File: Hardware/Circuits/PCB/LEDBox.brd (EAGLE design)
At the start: 28 x 28 mm, 19 parts

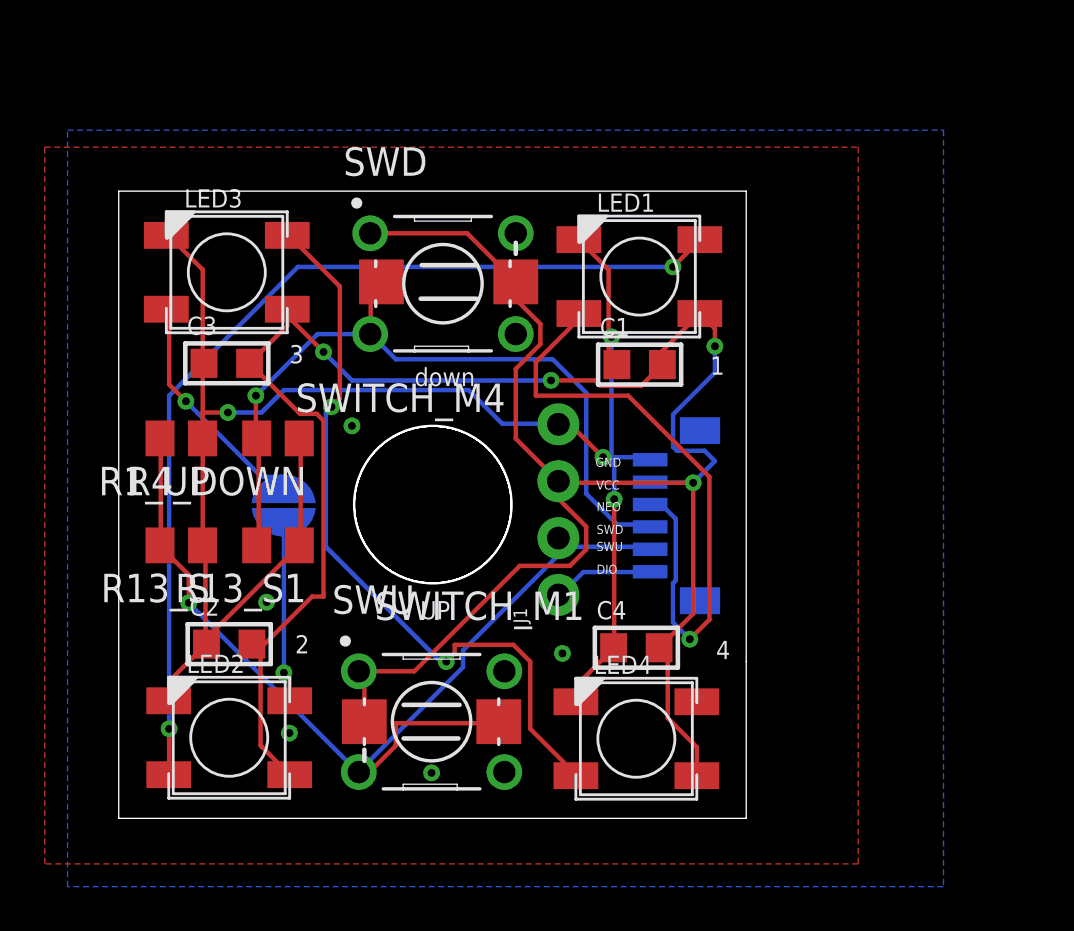
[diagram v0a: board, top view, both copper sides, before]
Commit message: update circuits
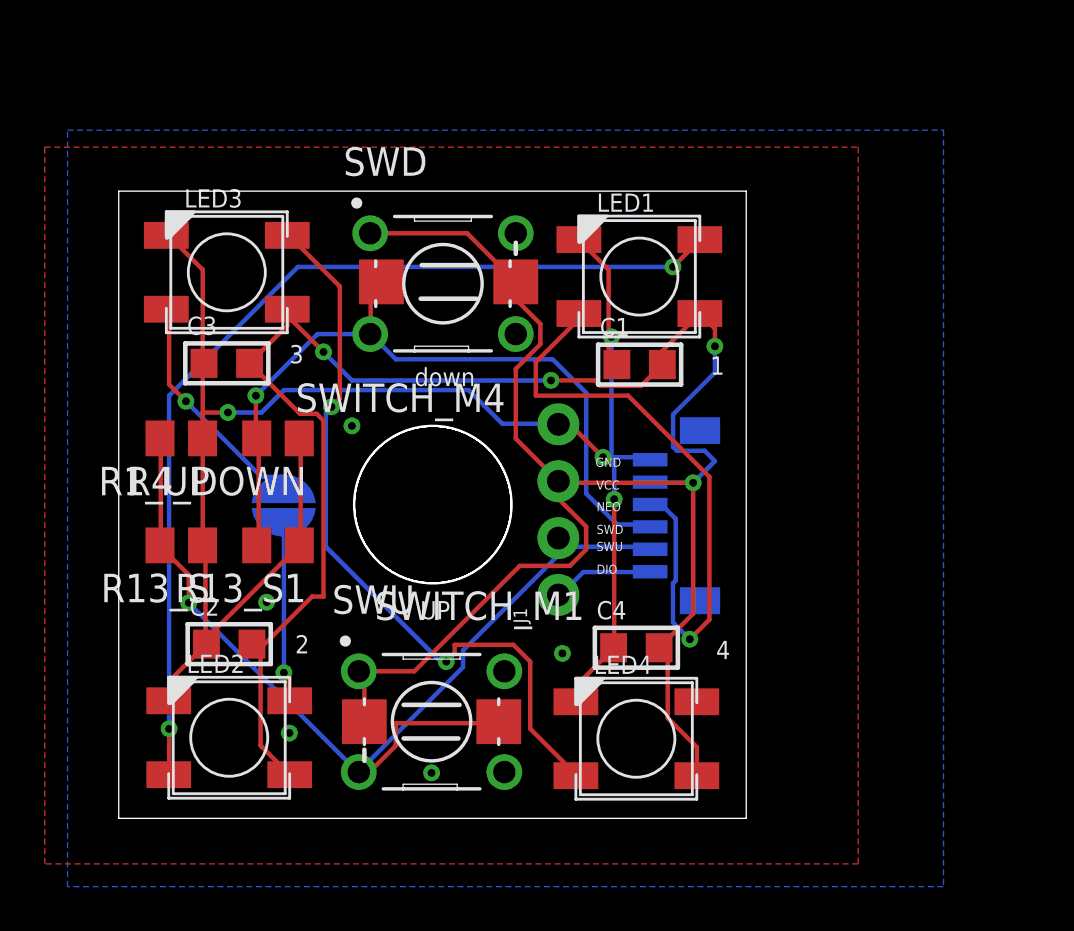
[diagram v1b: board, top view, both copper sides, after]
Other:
- outline, holes or cut-outs redrawn
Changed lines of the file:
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@@
 <drawing>
 <settings>
-<setting alwaysvectorfont="yes"/>
+<setting alwaysvectorfont="no"/>
 <setting verticaltext="up"/>
 </settings>
 <grid distance="10" unitdist="mil" unit="mm" style="lines" multiple="1" display="no" altdistance="1" altunitdist="mil" altunit="mm"/>
 <layers>
-<layer number="1" name="Top" color="4" fill="1" visible="yes" active="yes"/>
+<layer number="1" name="Top" color="4" fill="1" visible="no" active="yes"/>
 <layer number="2" name="Route2" color="16" fill="1" visible="no" active="no"/>
 <layer number="3" name="Route3" color="17" fill="1" visible="no" active="no"/>
@@
 <layer number="14" name="Route14" color="22" fill="1" visible="no" active="no"/>
 <layer number="15" name="Route15" color="23" fill="1" visible="no" active="no"/>
-<layer number="16" name="Bottom" color="1" fill="1" visible="yes" active="yes"/>
+<layer number="16" name="Bottom" color="1" fill="1" visible="no" active="yes"/>
 <layer number="17" name="Pads" color="2" fill="1" visible="yes" active="yes"/>
-<layer number="18" name="Vias" color="2" fill="1" visible="yes" active="yes"/>
-<layer number="19" name="Unrouted" color="6" fill="1" visible="yes" active="yes"/>
+<layer number="18" name="Vias" color="2" fill="1" visible="no" active="yes"/>
+<layer number="19" name="Unrouted" color="6" fill="1" visible="no" active="yes"/>
 <layer number="20" name="Dimension" color="24" fill="1" visible="yes" active="yes"/>
-<layer number="21" name="tPlace" color="7" fill="1" visible="yes" active="yes"/>
+<layer number="21" name="tPlace" color="7" fill="1" visible="no" active="yes"/>
 <layer number="22" name="bPlace" color="7" fill="1" visible="yes" active="yes"/>
-<layer number="23" name="tOrigins" color="15" fill="1" visible="yes" active="yes"/>
-<layer number="24" name="bOrigins" color="15" fill="1" visible="yes" active="yes"/>
-<layer number="25" name="tNames" color="7" fill="1" visible="yes" active="yes"/>
-<layer number="26" name="bNames" color="7" fill="1" visible="yes" active="yes"/>
+<layer number="23" name="tOrigins" color="15" fill="1" visible="no" active="yes"/>
+<layer number="24" name="bOrigins" color="15" fill="1" visible="no" active="yes"/>
+<layer number="25" name="tNames" color="7" fill="1" visible="no" active="yes"/>
+<layer number="26" name="bNames" color="7" fill="1" visible="no" active="yes"/>
 <layer number="27" name="tValues" color="7" fill="1" visible="no" active="yes"/>
 <layer number="28" name="bValues" color="7" fill="1" visible="no" active="yes"/>
@@
 <layer number="43" name="vRestrict" color="2" fill="10" visible="no" active="yes"/>
 <layer number="44" name="Drills" color="7" fill="1" visible="no" active="yes"/>
-<layer number="45" name="Holes" color="7" fill="1" visible="no" active="yes"/>
+<layer number="45" name="Holes" color="7" fill="1" visible="yes" active="yes"/>
 <layer number="46" name="Milling" color="3" fill="1" visible="no" active="yes"/>
 <layer number="47" name="Measures" color="7" fill="1" visible="no" active="yes"/>
-<layer number="48" name="Document" color="7" fill="1" visible="no" active="yes"/>
+<layer number="48" name="Document" color="7" fill="1" visible="yes" active="yes"/>
 <layer number="49" name="Reference" color="7" fill="1" visible="no" active="yes"/>
 <layer number="50" name="dxf" color="7" fill="1" visible="no" active="no"/>
@@
 <text x="21.336" y="10.922" size="0.4064" layer="21">DIO</text>
 <text x="13.462" y="8.89" size="0.8128" layer="21">UP</text>
-<wire x1="28.021" y1="28.009" x2="28.021" y2="7.009" width="0.01" layer="20"/>
-<wire x1="28.021" y1="7.009" x2="28.021" y2="0" width="0.01" layer="20"/>
+<wire x1="28.021" y1="28.009" x2="28.021" y2="0" width="0.01" layer="20"/>
 <wire x1="28.021" y1="0" x2="0" y2="0" width="0.01" layer="20"/>
 <wire x1="0" y1="0" x2="0" y2="28.009" width="0.01" layer="20"/>
@@
 <circle x="14.026" y="14.011" radius="3.5" width="0.01" layer="20"/>
 <circle x="14.026" y="14.011" radius="3.54" width="0.01" layer="20"/>
+<circle x="19.5834" y="17.5768" radius="0.915809375" width="0.001" layer="48"/>
+<circle x="19.5834" y="15.0368" radius="0.915809375" width="0.001" layer="48"/>
+<circle x="19.5834" y="12.4968" radius="0.915809375" width="0.001" layer="48"/>
+<circle x="19.5834" y="9.9568" radius="0.915809375" width="0.001" layer="48"/>
 </plain>
 <attributes>

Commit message: update motors
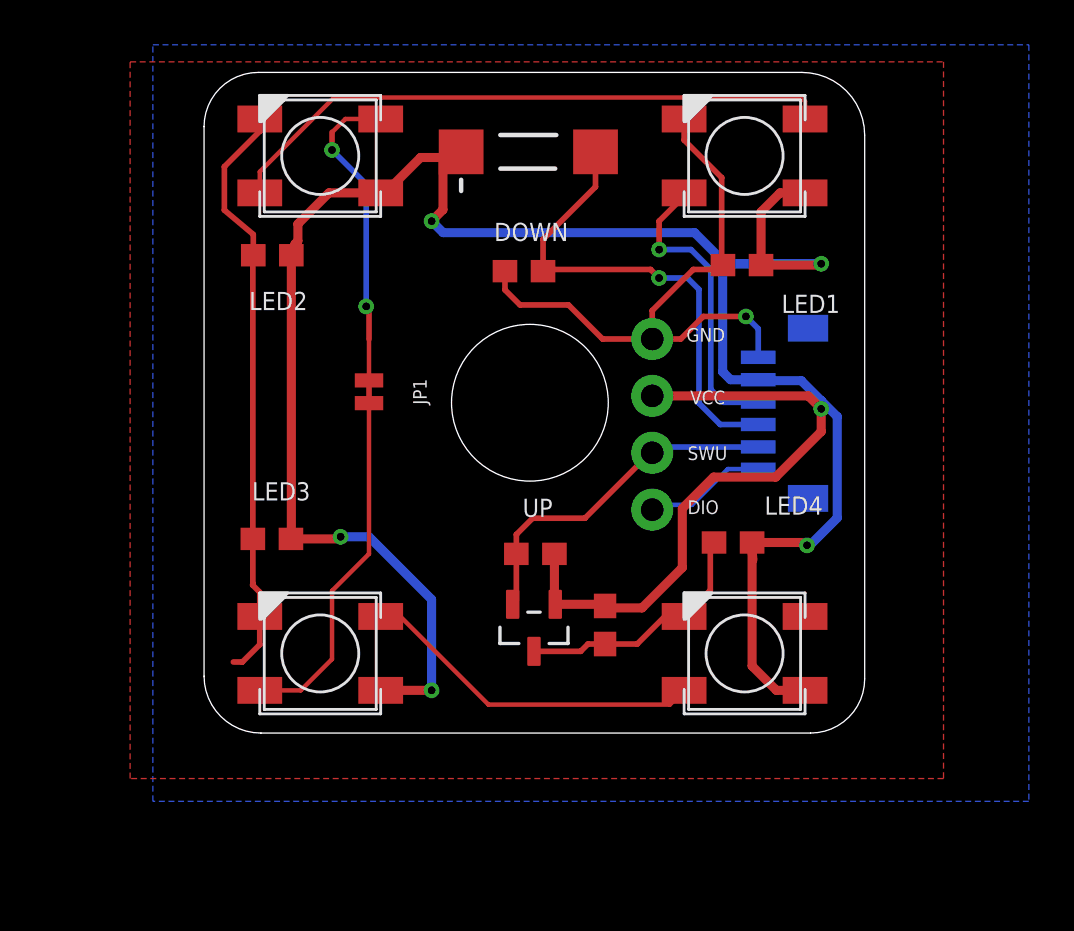
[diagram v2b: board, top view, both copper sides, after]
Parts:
- removed R13_S, R13_S1, R1_UP: 10K, resistor:M0805
- removed SWD, SWU: B3F-1000, Switch:B3F-1000
- removed SWITCH_M1: DTSM-3, switch-tact:DTSM-3
- added C5: 0.1uF, SparkFun-Capacitors:0603
- added R4_DOWN1: 10k, SparkFun-Resistors:0603
- added U1: TEXAS_INSTRUMENTS_DRV5033FAQDBZRTEXAS_INSTRUMENTS_DRV5033FA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, Texas Instruments - DRV5033FAQDBZR:TEXAS_INSTRUMENTS_DRV5033FAQDBZR_0
- C1, C2, C3, C4: value 0.1uf -> 0.1uF; device rc-master-smd:C0805 -> SparkFun-Capacitors:0603
- JP1: value JUMPER-SMT_2_NO_NO-SILK_ROUND -> LED; device SparkFun-Jumpers:SMT-JUMPER_2_NO_NO-SILK_ROUND -> SparkFun-Jumpers:SMT-JUMPER_2_NC_TRACE_NO-SILK
- R4_DOWN: value 10K -> 10k; device resistor:M0805 -> SparkFun-Resistors:0603
- moved LED2 26.3 mm to (9.00, 29.6)
- moved LED3 17.5 mm to (9.00, 7.37)
- moved R4_DOWN 13.3 mm to (18.1, 24.4), turned to 0 degrees
- moved LED1 7.15 mm to (27.9, 29.6)
- moved SWITCH_M4 6.81 mm to (18.3, 29.8), turned to 0 degrees
- moved J2 6.65 mm to (29.8, 18.0)
- moved C4 6.38 mm to (27.4, 12.3)
- moved C1 6.38 mm to (27.8, 24.7)
- moved JP1 6.35 mm to (11.2, 19.1), flipped to the top, turned to 270 degrees
- moved LED4 6.15 mm to (27.9, 7.37)
- moved J1 5.66 mm to (23.8, 13.8)
- moved C3 5.24 mm to (6.86, 25.1)
- moved C2 5.07 mm to (6.84, 12.5)
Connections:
- net GND: now also C5.1, U1.3; no longer R13_S.1, R13_S1.1, R1_UP.1
- net SWD_IN: no longer R13_S1.2, SWD.3
- net SWU_IN: now also R4_DOWN1.2, U1.2; no longer R13_S.2, R1_UP.2, SWITCH_M1.2, SWU.3
- net VCC: now also C5.2, R4_DOWN1.1, U1.1; no longer SWD.1, SWITCH_M1.1, SWU.1
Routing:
- net SWU_IN: track 45.1 -> 15.6 mm, vias 1 -> 0
- net N$6: track 33.2 -> 15.4 mm, vias 2 -> 0
- net N$1: track 43.5 -> 27.5 mm, vias 2 -> 0
- net NEO_IN: track 28.5 -> 13.4 mm
- net GND: track 78.4 -> 65.3 mm, vias 9 -> 1
- net SWD_IN: track 34.3 -> 21.8 mm
- net VCC: track 116.7 -> 127.8 mm, vias 4 -> 6
- net N$2: track 7.56 -> 14.7 mm, vias 1 -> 2
- net N$4: track 10.2 -> 15.9 mm, vias 1 -> 0
- net DIO_IN: track 4.52 -> 5.48 mm
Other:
- board size 28 x 28 mm -> 29.5 x 29.5 mm
- board text added: "+"
- board text added: "-"
- board text added: "DOWN"
- board text removed: "1"
- board text removed: "2"
- board text removed: "3"
- board text removed: "4"
- board text removed: "SWD"
- board text removed: "down"
